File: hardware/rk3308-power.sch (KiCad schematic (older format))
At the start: 25 parts, among them Q1 BSS138, SW1 SW_SKSC_4PIN, U1000 RK3308, Y2 Crystal_GND24

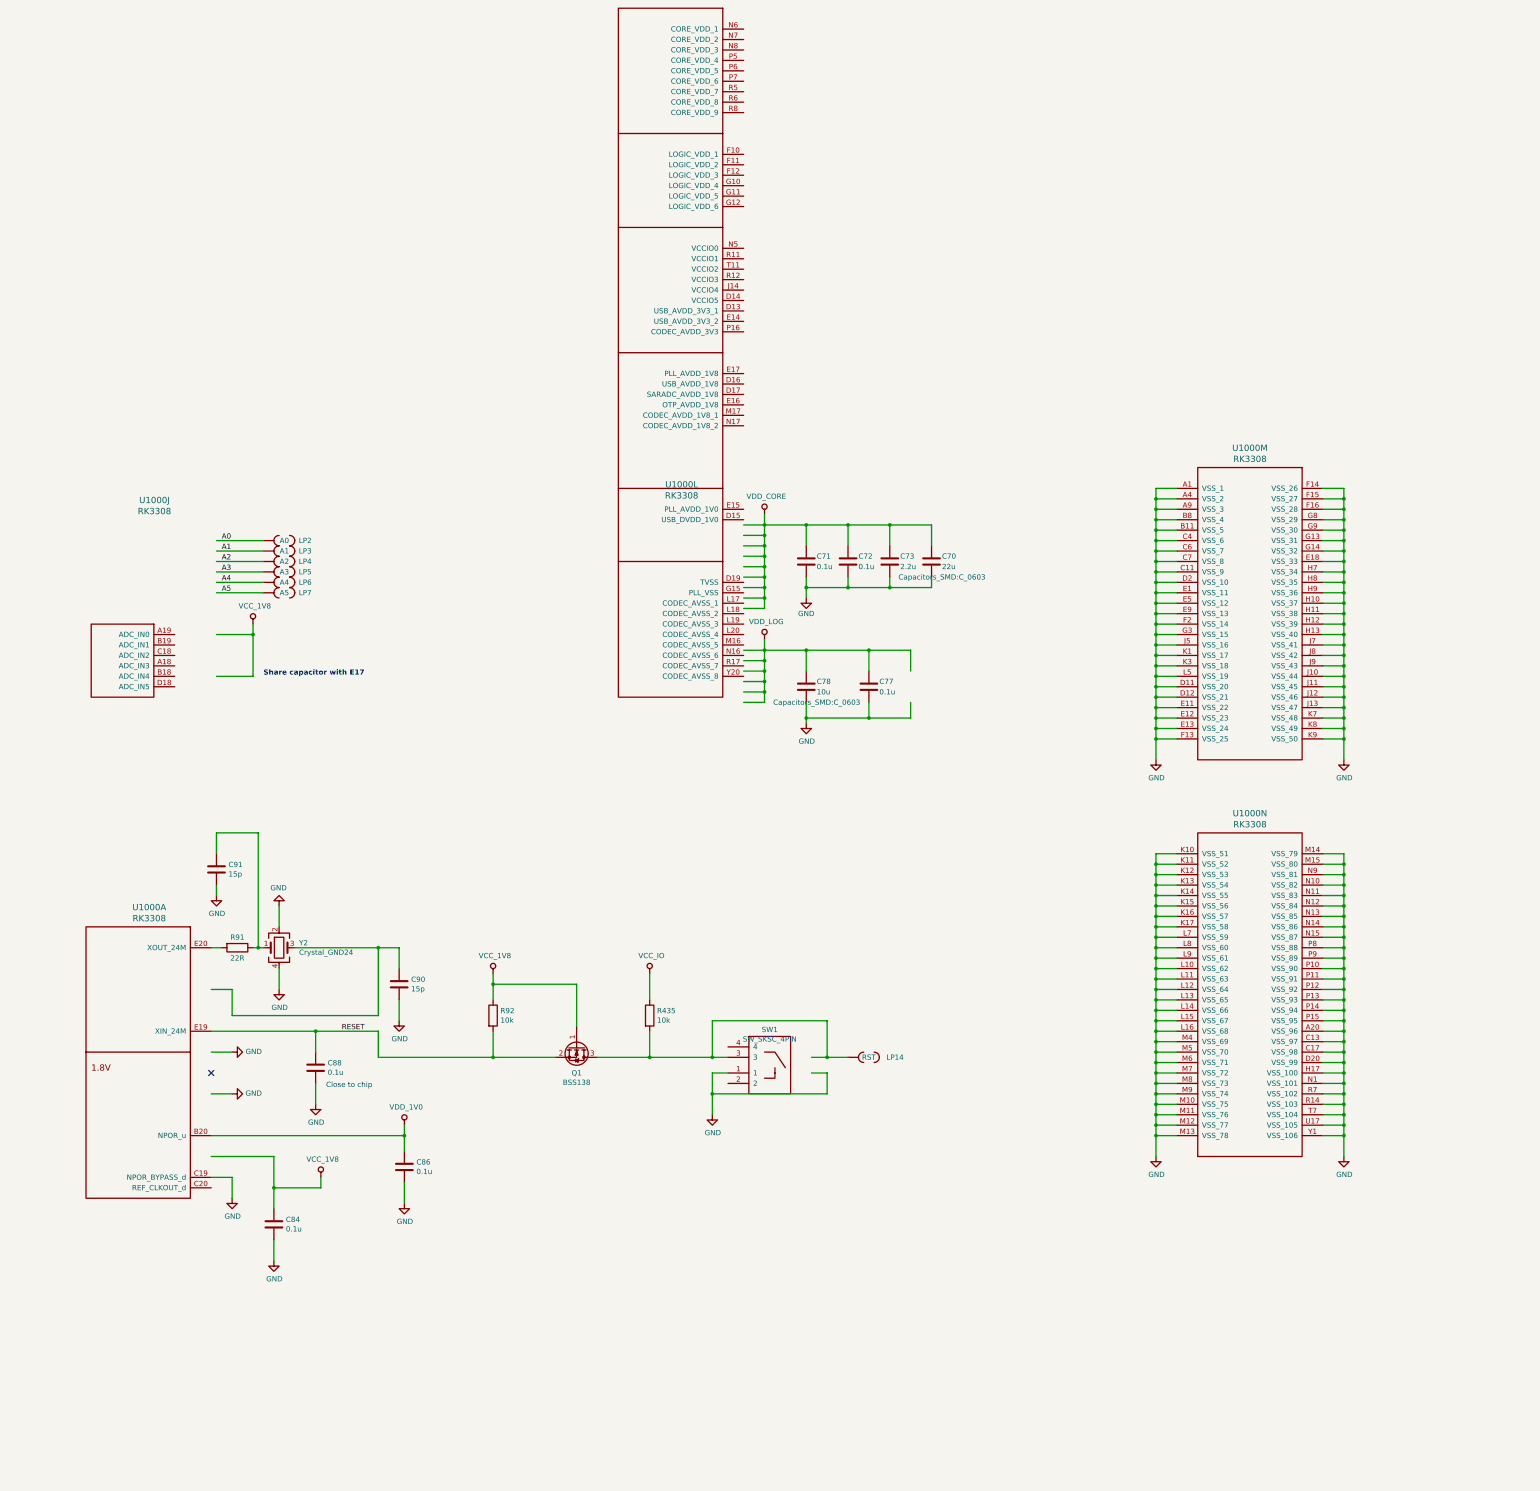
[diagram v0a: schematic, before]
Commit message: wip
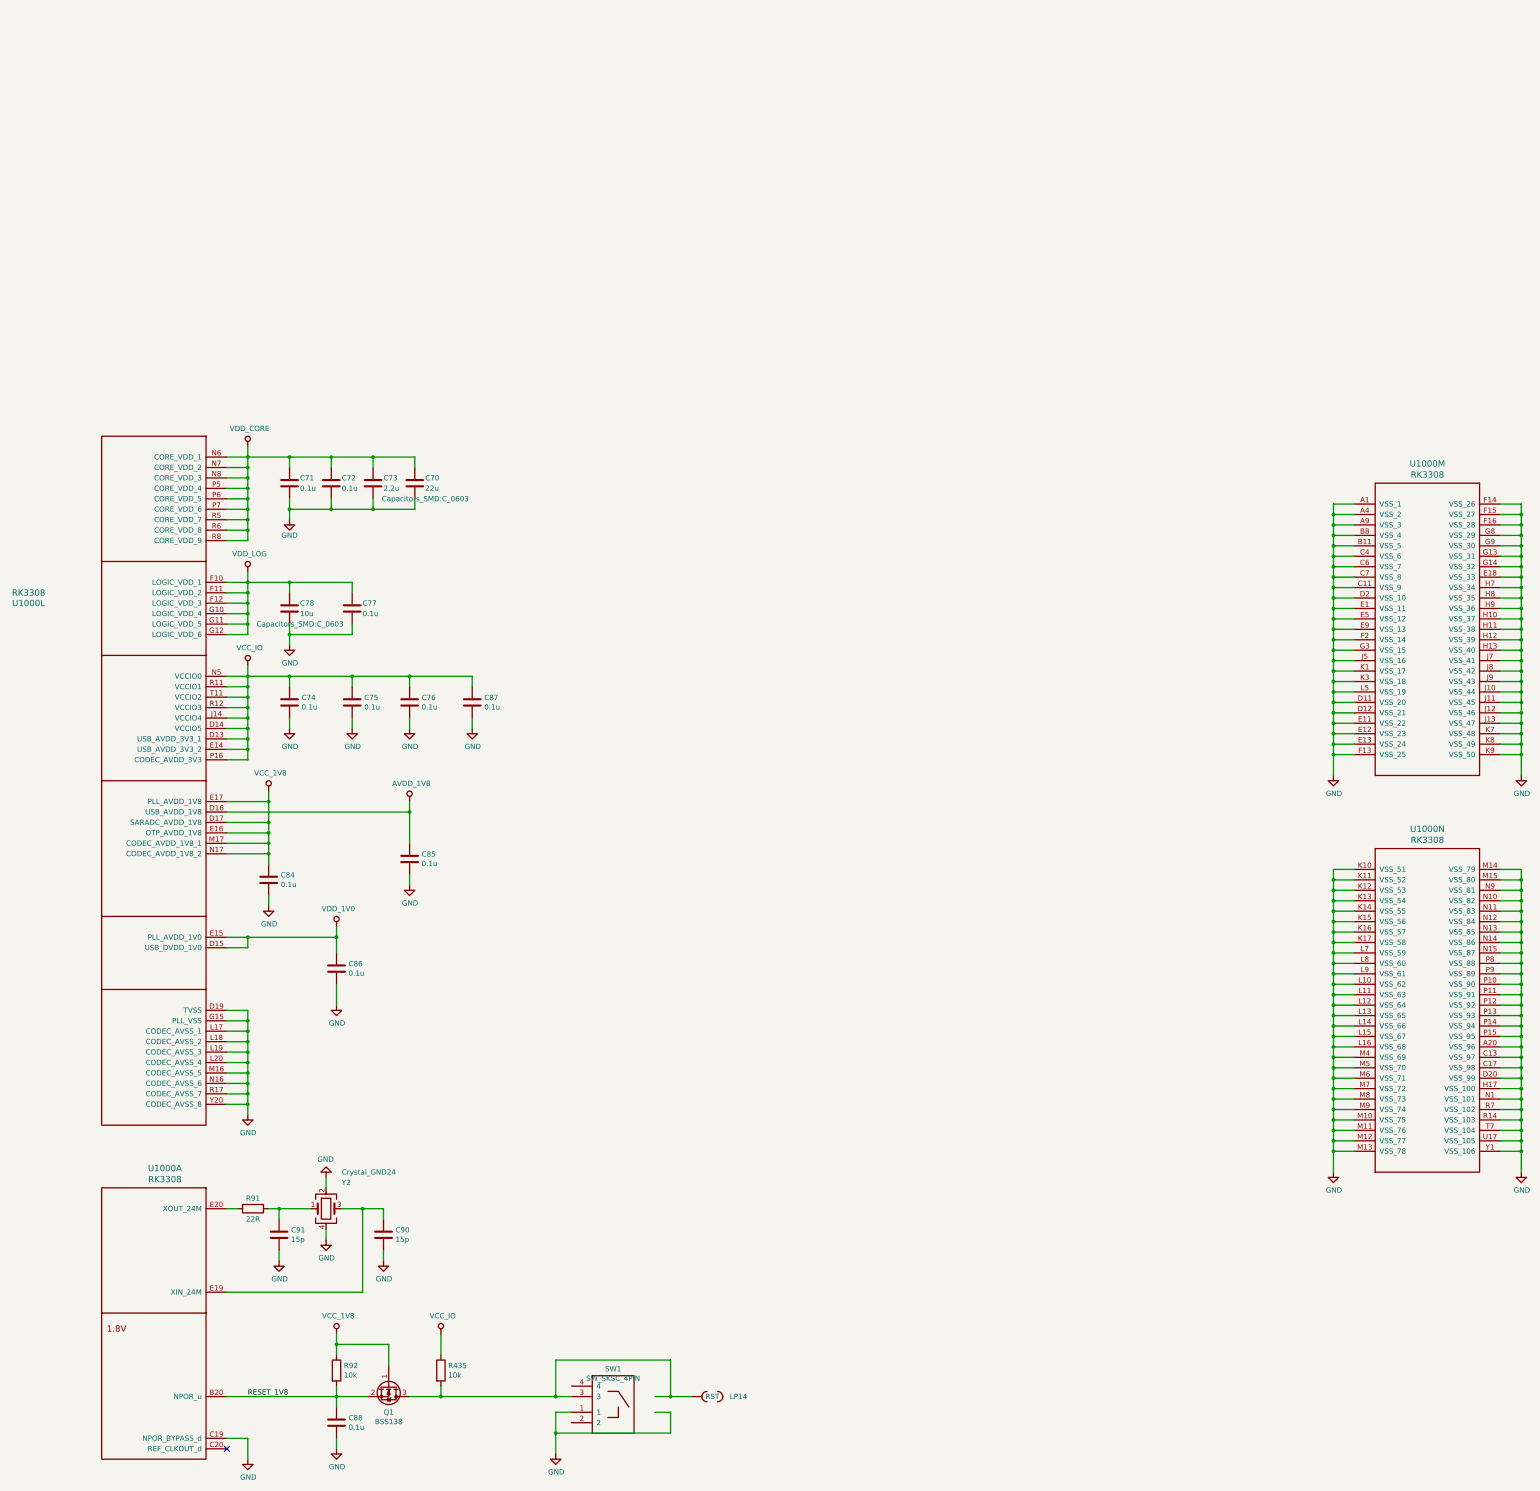
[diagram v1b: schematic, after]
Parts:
- removed LP2: A0, require:OVAL_PIN, symbol require:OP
- removed LP3: A1, require:OVAL_PIN, symbol require:OP
- removed LP4: A2, require:OVAL_PIN, symbol require:OP
- removed LP5: A3, require:OVAL_PIN, symbol require:OP
- removed LP6: A4, require:OVAL_PIN, symbol require:OP
- removed LP7: A5, require:OVAL_PIN, symbol require:OP
- removed unit 10 of U1000
- added C74, C75, C76, C85, C87: 0.1u, Capacitors_SMD:C_0402, symbol Device:C
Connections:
- net labels added: AVDD_1V8, RESET_1V8
- net labels removed: A0, A1, A2, A3, A4, A5, RESET
- wire segments 339 -> 379
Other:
- note removed: "Close to chip"
- note removed: "Share capacitor with E17"
- moved on the sheet: C70, C71, C72, C73, C77, C78, C84, C86, C88, C90, C91, LP14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

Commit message: wip
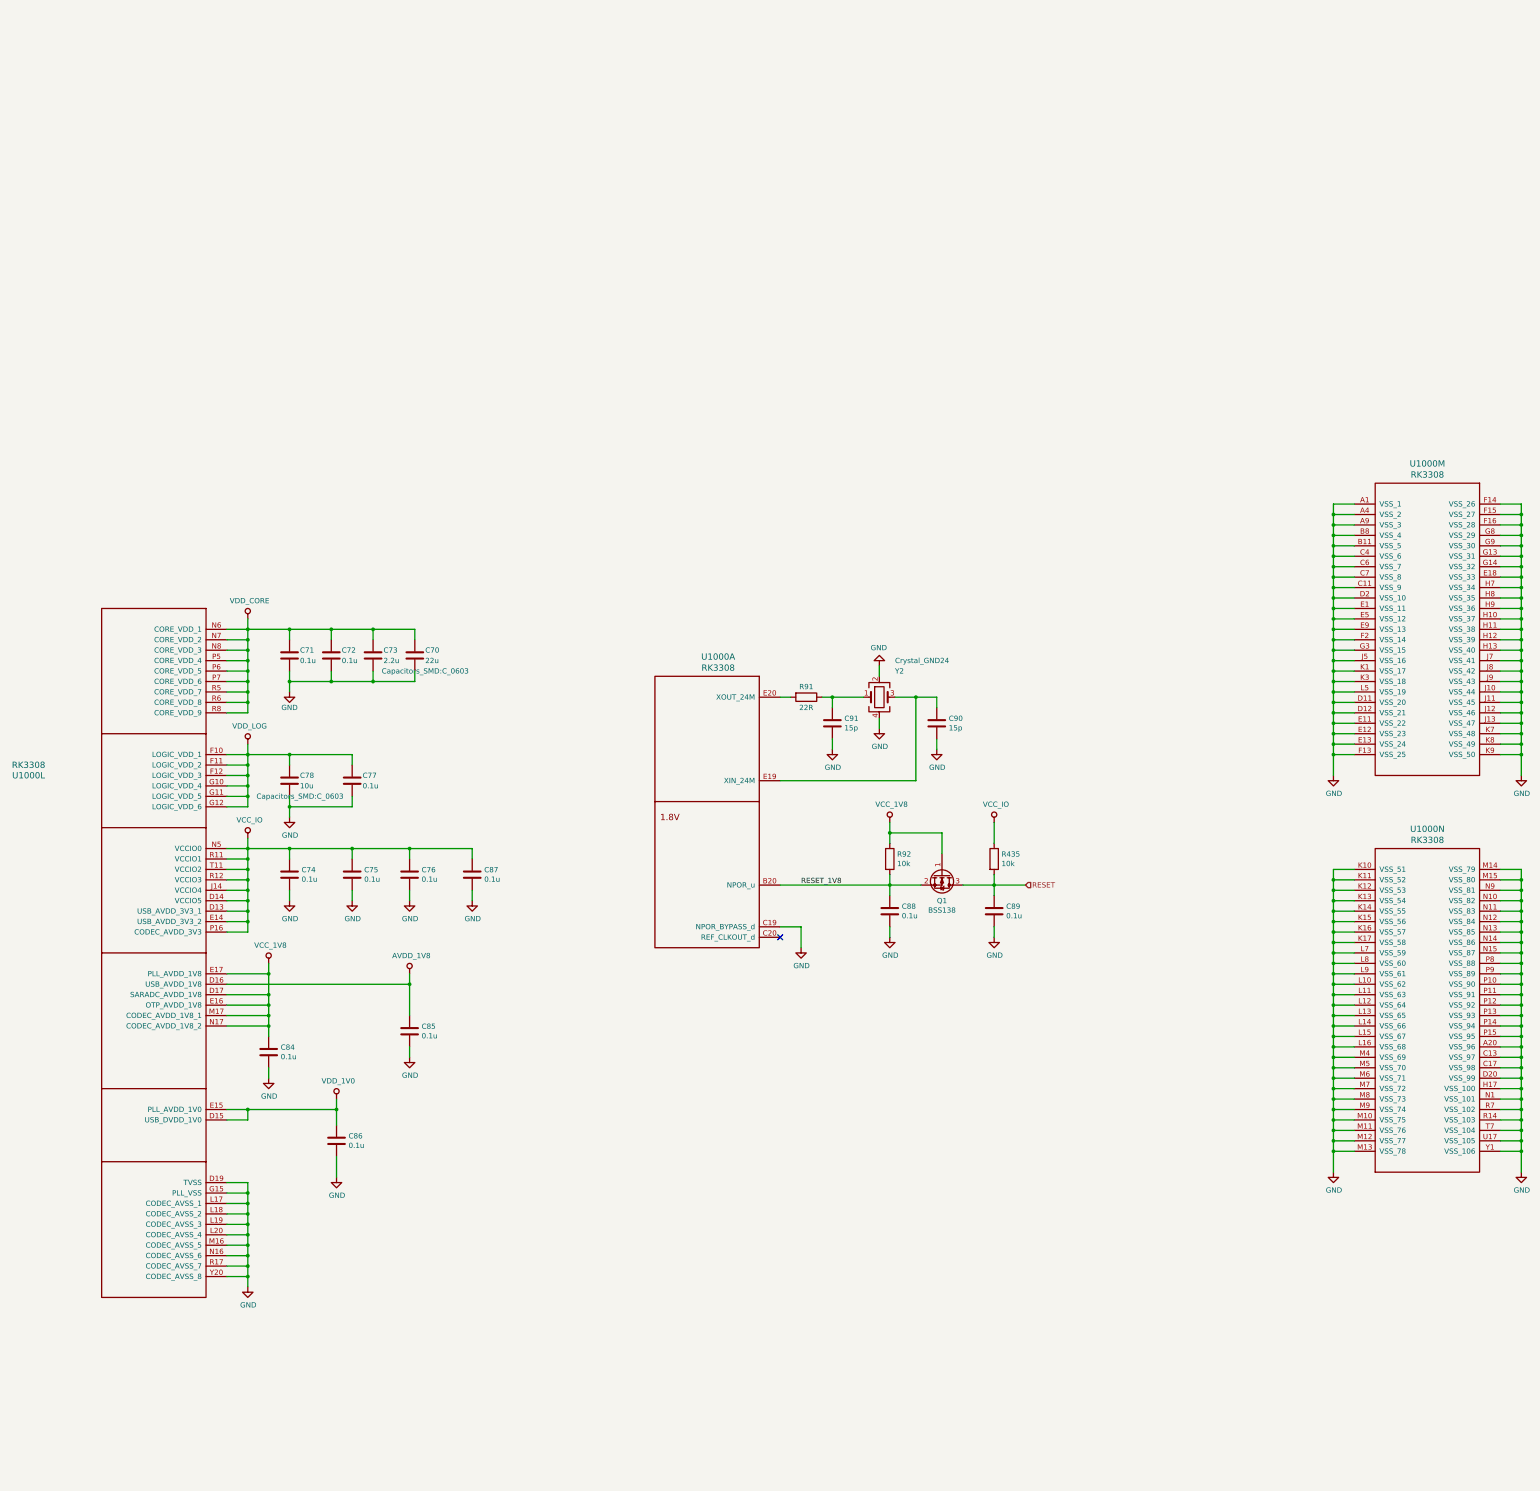
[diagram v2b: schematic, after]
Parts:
- removed LP14: RST, require:OVAL_PIN, symbol require:OP
- removed SW1: SW_SKSC_4PIN, require:SW_ALPS_SKSC, symbol require:SW_SKSC_4PIN
- added C89: 0.1u, Capacitors_SMD:C_0402, symbol Device:C
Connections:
- net GND: now also C89.2
- net RESET: now reaches Q1.3 (D), R435.2
- net RESET: now also C89.1
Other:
- moved on the sheet: C70, C71, C72, C73, C74, C75, C76, C77, C78, C84, C85, C86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
